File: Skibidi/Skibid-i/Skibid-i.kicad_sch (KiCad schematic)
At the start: 53 parts, among them IC1 TEENSY_4.1, J1 XT60-M, J10 Screw_Terminal_01x04, J11 Screw_Terminal_01x04, J12 Screw_Terminal_01x03, J13 Screw_Terminal_01x03, J14 XT60-M, J15 Conn_01x03_Pin, J16 XT60-M, J18 Sparkin, J19 Sparkout, J2 XT60-M, J21 Motor1, J22 Motor2, J3 Screw_Terminal_01x03, J4 Screw_Terminal_01x03, J5 Screw_Terminal_01x03, J6 Screw_Terminal_01x03, J7 Screw_Terminal_01x03, J8 Screw_Terminal_01x03, J9 Screw_Terminal_01x03, SW1 500SSP1S2M2QEA, U1 LTV-827S, U2 LTV-827S, U3 LTV-827S, U4 LTV-827S, U5 LTV-827S, U6 LTV-827S, U7 LTV-827S

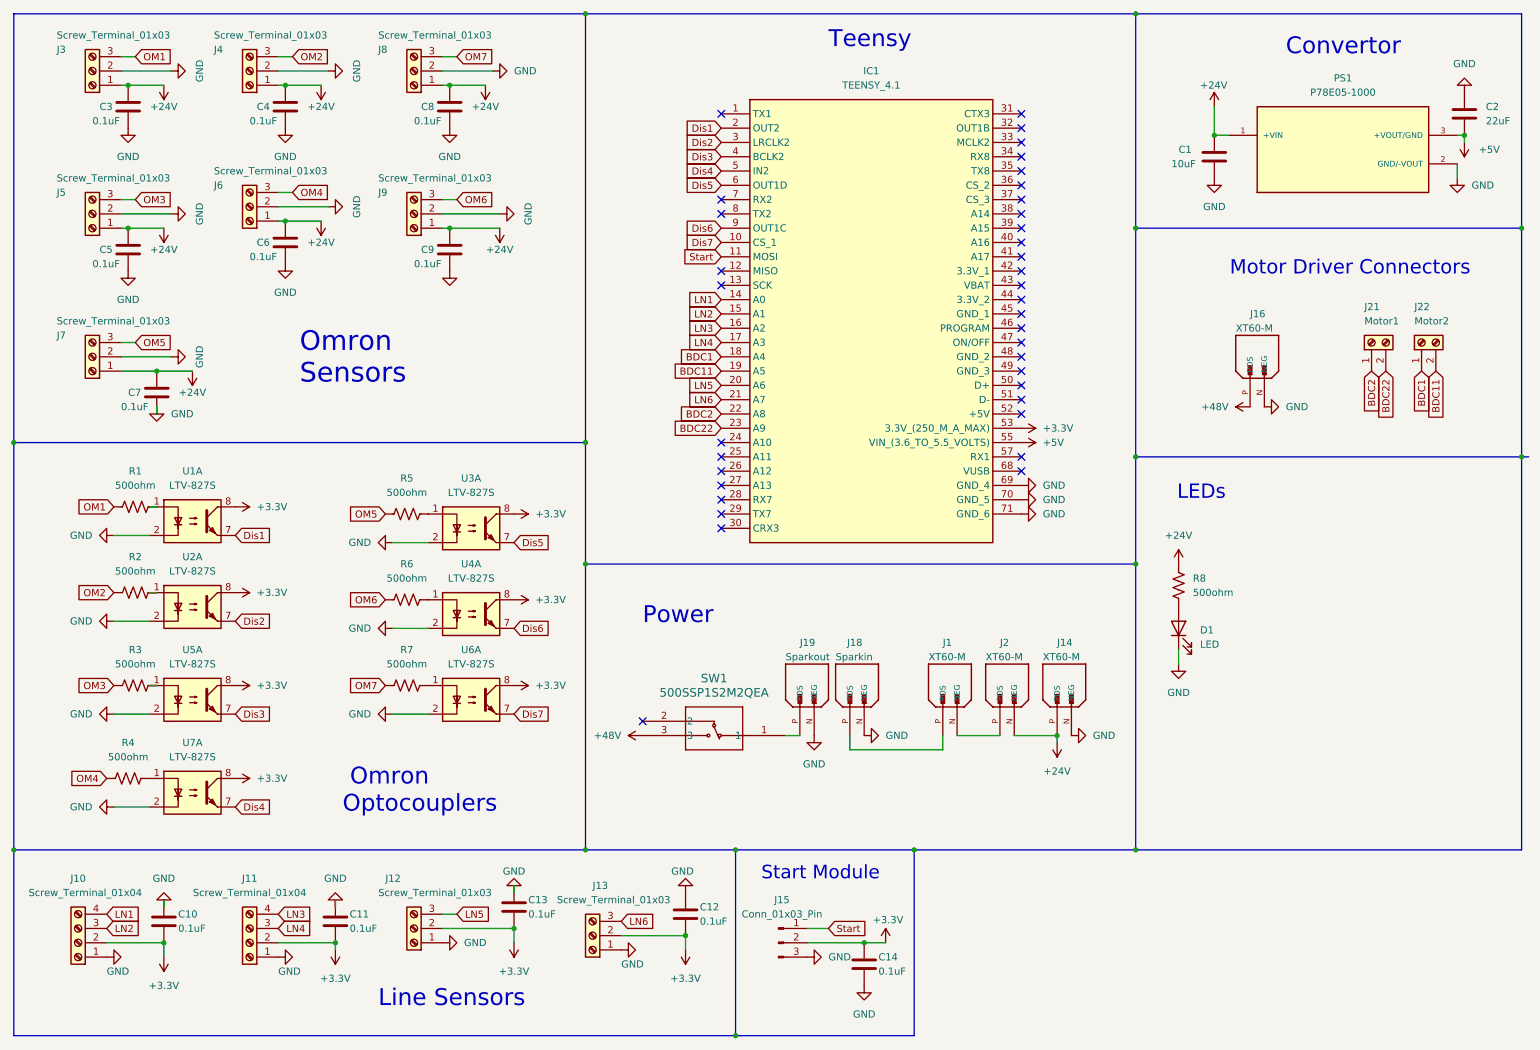
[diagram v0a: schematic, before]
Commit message: added foortprints
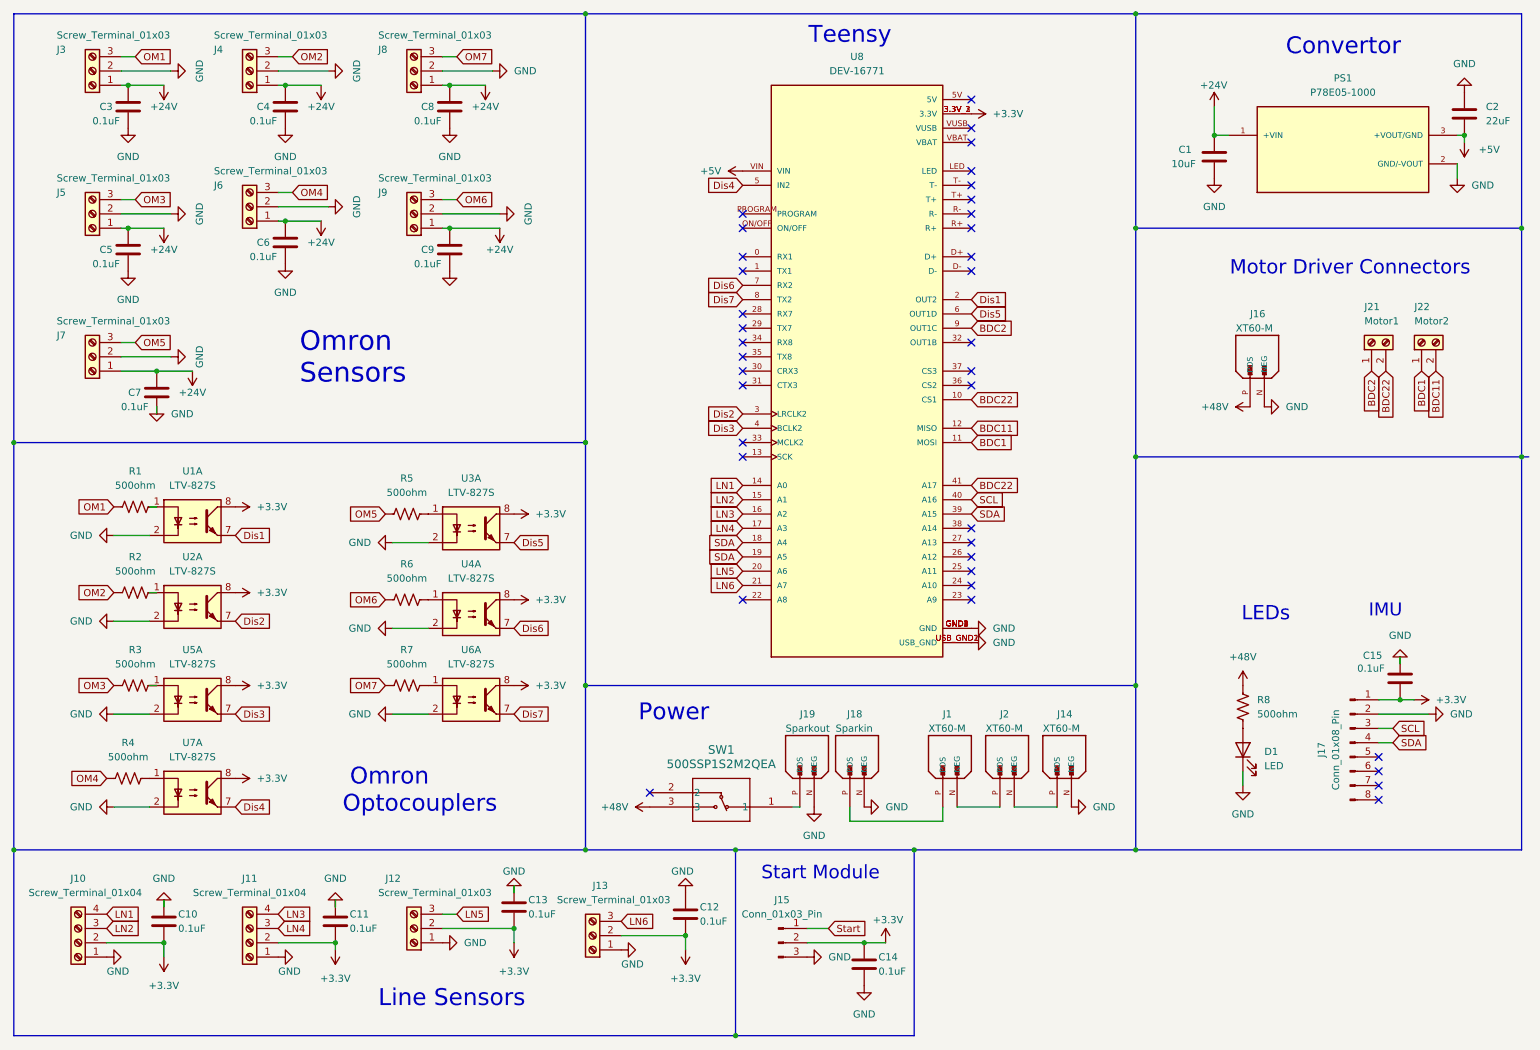
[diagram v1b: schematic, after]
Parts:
- removed IC1: TEENSY_4.1, TEENSY41, symbol TEENSY_4_1:TEENSY_4.1
- added C15: 0.1uF, Skibidi-feet:C_0805_2012Metric, symbol Device:C
- added J17: Conn_01x08_Pin, Connector_PinHeader_2.54mm:PinHeader_1x08_P2.54mm_Vertical, symbol Connector:Conn_01x08_Pin
- added U8: DEV-16771, Skibidi-feet:TEENSY, symbol Teensy4.1:DEV-16771
- C10, C11, C12, C13, C14, C3, C4, C5, C6, C7, C8, C9: footprint (none) -> Skibidi-feet:C_0805_2012Metric
- D1: footprint (none) -> Skibidi-feet:LED
- J1, J14, J16, J18, J19, J2: footprint XT60-M:AMASS_XT60-M -> Skibidi-feet:XT60
- J12, J13, J3, J4, J5, J6, J7, J8, J9: footprint (none) -> Skibidi-feet:ScrewTerminal3
- J15: footprint (none) -> Connector_PinHeader_2.54mm:PinHeader_1x03_P2.54mm_Vertical
- PS1: footprint P78E05-1000:CONV_P78E05-1000 -> Skibidi-feet:5vConvertor
- R1, R2, R3, R4, R5, R6, R7, R8: footprint (none) -> Resistor_SMD:R_0805_2012Metric
- SW1: footprint THERAPI:SWITCH -> Skibidi-feet:SWitch
- U1, U2, U3, U4, U5, U6, U7: footprint Package_DIP:SMDIP-8_W9.53mm -> Skibidi-feet:Optocoupler
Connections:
- net +24V: no longer J14.P (POS), J2.N (NEG), R8.2
- net +3.3V: now also C15.2, J17.1 (Pin_1), U8.3.3V_1 (3.3V), U8.3.3V_2 (3.3V), U8.3.3V_3 (3.3V)
- net +48V: now also R8.2
- net +5V: now also U8.VIN
- net BDC1: now also U8.11 (MOSI)
- net BDC11: now also U8.12 (MISO)
- net BDC2: now also U8.9 (OUT1C)
- net BDC22: now also U8.10 (CS1), U8.41 (A17)
- net Dis1: now also U8.2 (OUT2)
- net Dis2: now also U8.3 (LRCLK2)
- net Dis3: now also U8.4 (BCLK2)
- net Dis4: now also U8.5 (IN2)
- net Dis5: now also U8.6 (OUT1D)
- net Dis6: now also U8.7 (RX2)
- net Dis7: now also U8.8 (TX2)
- net GND: now also C15.1, J17.2 (Pin_2), U8.GND1 (GND), U8.GND2 (GND), U8.GND3 (GND), U8.GND4 (GND), U8.GND5 (GND), U8.USB_GND1 (USB_GND), U8.USB_GND2 (USB_GND)
- net LN1: now also U8.14 (A0)
- net LN2: now also U8.15 (A1)
- net LN3: now also U8.16 (A2)
- net LN4: now also U8.17 (A3)
- net LN5: now also U8.20 (A6)
- net LN6: now also U8.21 (A7)
- new net: J14.P (POS), J2.N (NEG)
- new net SCL: J17.3 (Pin_3), U8.40 (A16)
- new net SDA: J17.4 (Pin_4), U8.18 (A4), U8.19 (A5), U8.39 (A15)
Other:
- note added: "IMU"
- moved on the sheet: D1, J1, J14, J18, J19, J2, R8, SW1
